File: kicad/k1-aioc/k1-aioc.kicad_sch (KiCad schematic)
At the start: 46 parts, among them J1 12401832E402A, J2 Conn_01x07_Male, Q1 BC847BS, U1 TLV1117LV-33, U2 STM32F373CBTx, U3 TLV1117LV-33, Y1 8MHz/20pF

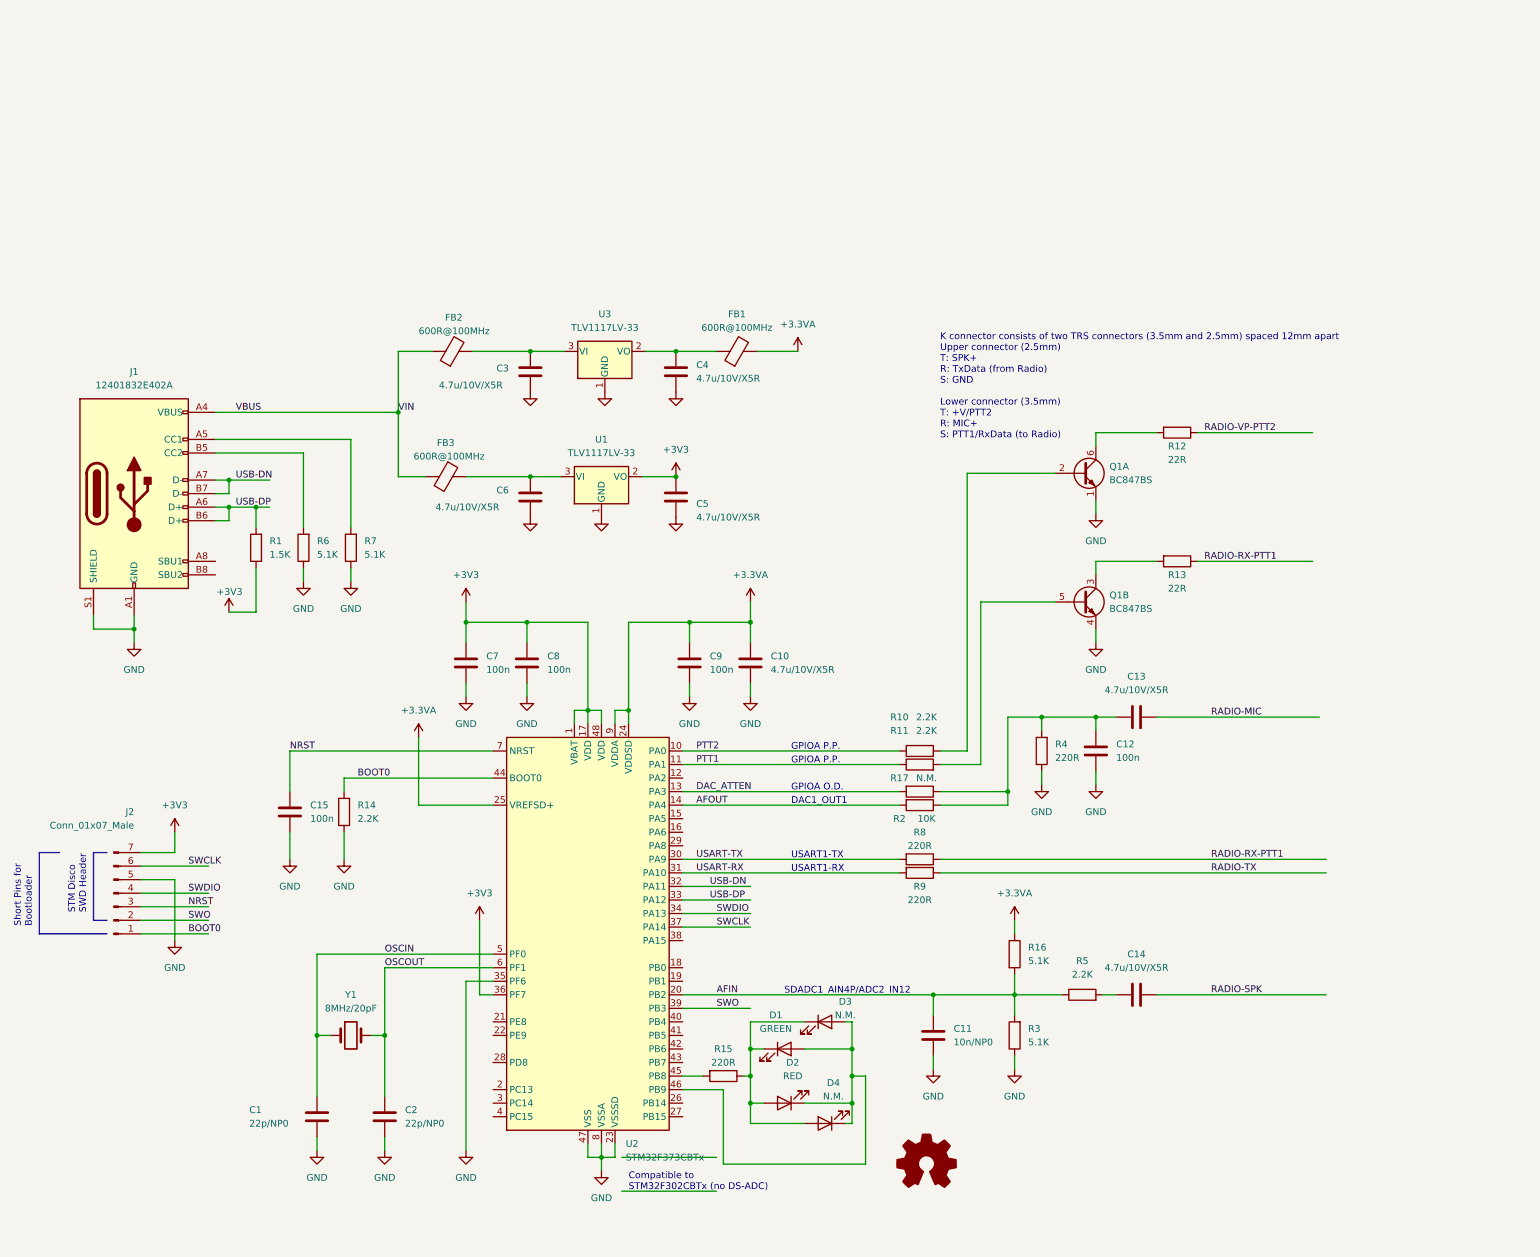
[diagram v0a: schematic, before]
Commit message: Adding USB isolation
- Isolated 5V DC/DC converter
- ADUM3160 USB Isolator
- 1.5k PU optional (handled by ADUM3160)
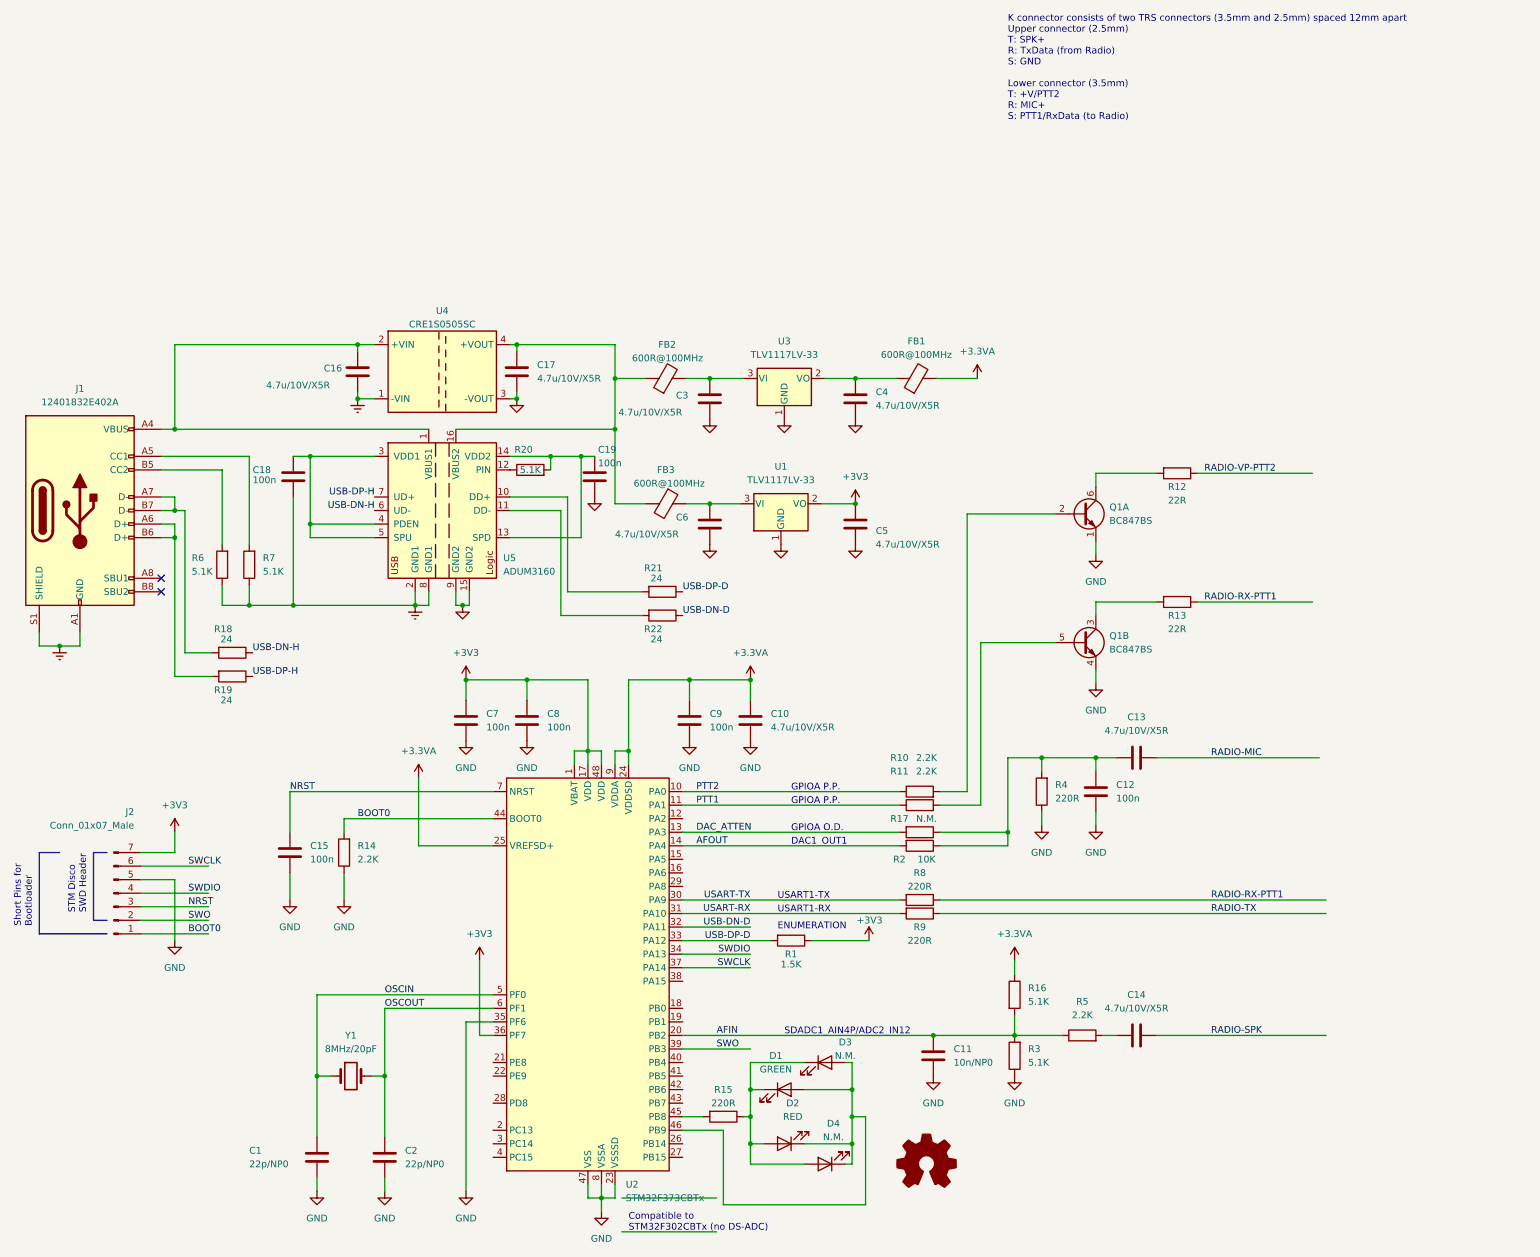
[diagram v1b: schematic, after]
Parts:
- added C16, C17: 4.7u/10V/X5R, Capacitor_SMD:C_0805_2012Metric, symbol Device:C
- added C18, C19: 100n, Capacitor_SMD:C_0805_2012Metric, symbol Device:C
- added R18, R19, R21, R22: 24, Resistor_SMD:R_0805_2012Metric, symbol Device:R
- added R20: 5.1K, Resistor_SMD:R_0805_2012Metric, symbol Device:R
- added U4: CRE1S0505SC, Converter_DCDC:Converter_DCDC_Murata_CRE1xxxxxxSC_THT, symbol Regulator_Switching:CRE1S0505SC
- added U5: ADUM3160, Package_SO:SOIC-16W_7.5x10.3mm_P1.27mm, symbol Interface_USB:ADUM3160
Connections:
- net GND: now also C17.2, C19.2, U4.3 (-VOUT), U5.15 (GND2), U5.9 (GND2); no longer J1.A1 (GND), J1.A12 (GND), J1.B1 (GND), J1.B12 (GND), J1.S1 (SHIELD), R6.1, R7.1
- net USB-DN: no longer names the net of J1.A7 (D-), J1.B7 (D-)
- net USB-DN: now also R18.2; no longer U2.32 (PA11)
- net USB-DP: no longer names the net of J1.A6 (D+), J1.B6 (D+)
- net USB-DP: now also R19.2; no longer R1.2, U2.33 (PA12)
- net VBUS: no longer names the net of J1.A4 (VBUS), J1.A9 (VBUS), J1.B4 (VBUS), J1.B9 (VBUS)
- net VBUS: now also C16.1, U4.2 (+VIN), U5.1 (VBUS1); no longer FB2.1, FB3.2
- new net: R21.2, U5.10 (DD+)
- new net: C17.1, FB2.1, FB3.2, U4.4 (+VOUT), U5.16 (VBUS2)
- new net: R22.2, U5.11 (DD-)
- new net: C19.1, R20.2, U5.13 (SPD), U5.14 (VDD2)
- new net: C18.1, U5.3 (VDD1), U5.4 (PDEN), U5.5 (SPU)
- new net: R20.1, U5.12 (PIN)
- new net GNDREF: C16.2, C18.2, J1.A1 (GND), J1.A12 (GND), J1.B1 (GND), J1.B12 (GND), J1.S1 (SHIELD), R6.1, R7.1, U4.1 (-VIN), U5.2 (GND1), U5.8 (GND1)
- new net USB-DN-D: R22.1, U2.32 (PA11)
- new net USB-DN-H: R18.1, U5.6 (UD-)
- new net USB-DP-D: R1.2, R21.1, U2.33 (PA12)
- new net USB-DP-H: R19.1, U5.7 (UD+)
- no-connect marks 0 -> 2
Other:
- note added: "ENUMERATION"
- moved on the sheet: C1, C10, C11, C12, C13, C14, C15, C2, C3, C4, C5, C6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
